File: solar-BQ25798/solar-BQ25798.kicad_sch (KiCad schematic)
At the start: 88 parts, among them J101 Power In, J102 Power OUT, J103 Power OUT, Q1 Q_NMOS_GSD, Q101 DMP4013LFGQ-13, Q102 2N7002, U101 HT75xx-1-SOT89, U102 INA219AxDCN

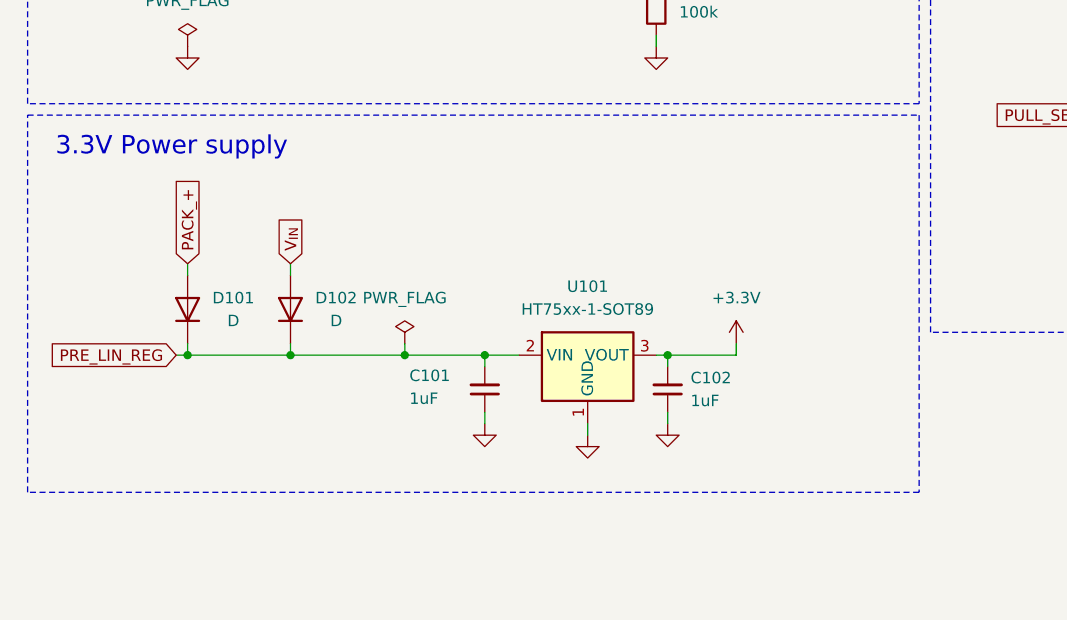
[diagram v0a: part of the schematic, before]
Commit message: Update buzzer and 3D files
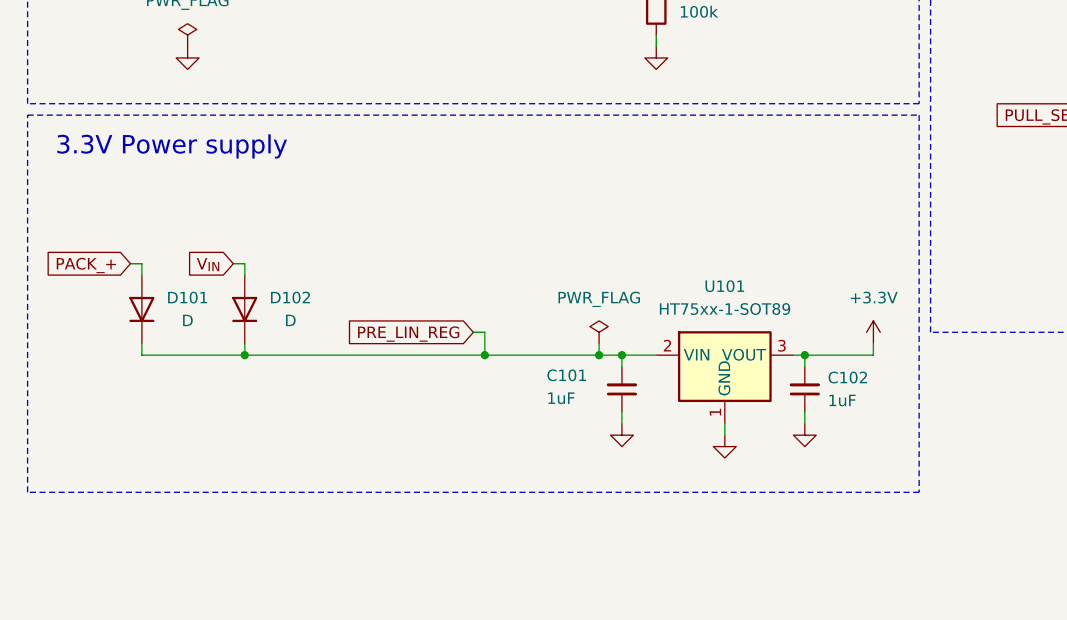
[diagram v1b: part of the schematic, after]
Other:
- moved on the sheet: C101, C102, D101, D102, U101
